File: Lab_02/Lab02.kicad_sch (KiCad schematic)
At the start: 0 parts

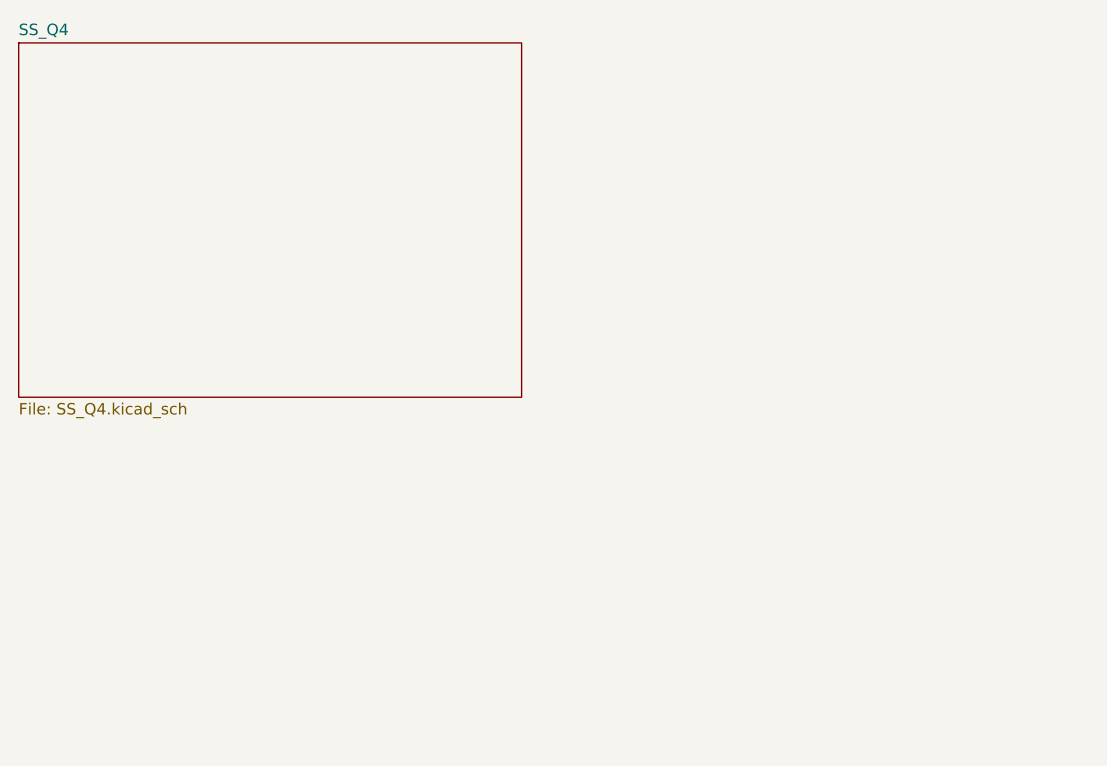
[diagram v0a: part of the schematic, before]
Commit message: q4 ss done
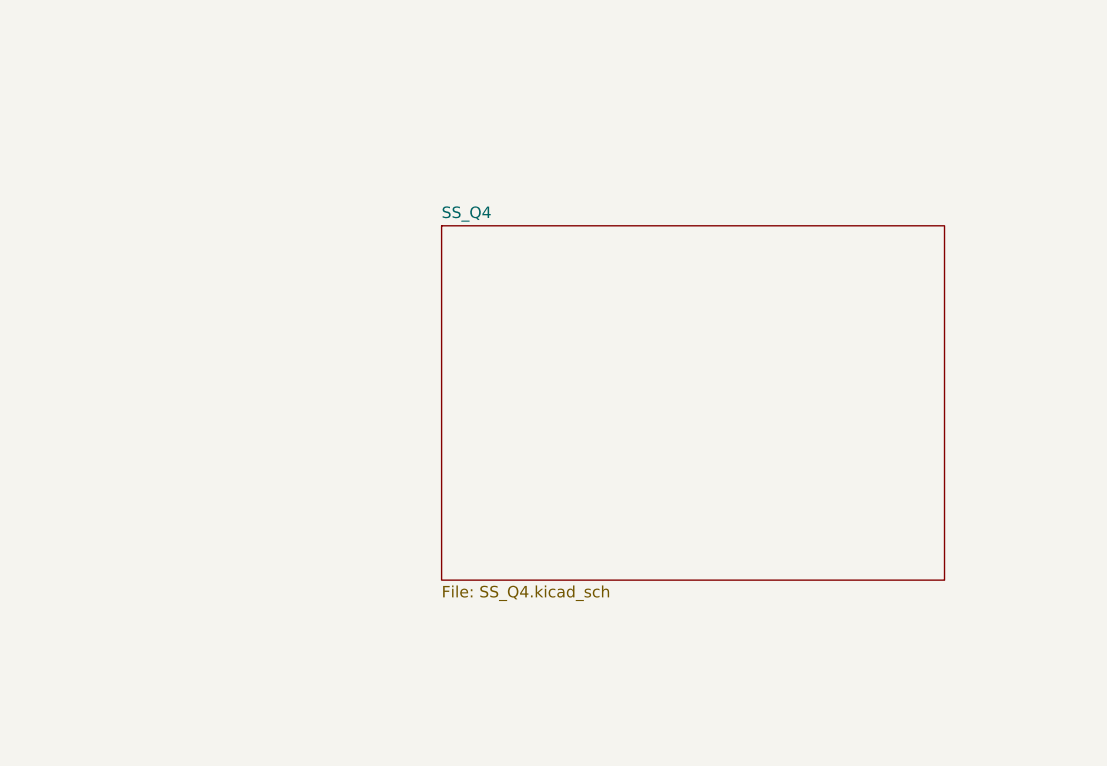
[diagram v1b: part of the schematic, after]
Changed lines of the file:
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@@
     )
   )
-  (sheet (at 40.64 35.56) (size 55.88 39.37) (fields_autoplaced)
+  (sheet (at 87.63 55.88) (size 55.88 39.37) (fields_autoplaced)
     (stroke (width 0.1524) (type solid))
     (fill (color 0 0 0 0.0000))
-    (property "Sheetname" "SS_Q4" (at 40.64 34.8484 0)
+    (property "Sheetname" "SS_Q4" (at 87.63 55.1684 0)
       (effects (font (size 1.27 1.27)) (justify left bottom))
     )
-    (property "Sheetfile" "SS_Q4.kicad_sch" (at 40.64 75.5146 0)
+    (property "Sheetfile" "SS_Q4.kicad_sch" (at 87.63 95.8346 0)
       (effects (font (size 1.27 1.27)) (justify left top))
     )
